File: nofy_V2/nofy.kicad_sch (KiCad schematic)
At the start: 144 parts, among them J10 Conn_01x01-Connector_Generic, J11 Conn_01x01-Connector_Generic, J12 Conn_01x01-Connector_Generic, J13 Conn_01x01-Connector_Generic, J14 Conn_01x01-Connector_Generic, J15 Conn_01x01-Connector_Generic, J16 Conn_01x01-Connector_Generic, J17 Conn_01x01-Connector_Generic, J18 Conn_01x01-Connector_Generic, J19 Conn_01x01-Connector_Generic, J20 Conn_01x01-Connector_Generic, J21 Conn_01x01-Connector_Generic, J22 PIn1x4, J23 PIn1x4, J24 PIn1x4, J25 PIn1x4, J26 PIn1x4, J27 PIn1x4, J28 PIn1x4, J29 PIn1x4, J30 PIn1x4, J31 PIn1x4, J32 PIn1x4, J33 PIn1x4, J34 PIn1x4, J35 PIn1x4, J36 PIn1x4, J37 PIn1x4, J38 PIn1x4, J39 PIn1x4, J40 PIn1x4, J41 PIn1x4, SW1 RotaryEncoder, SW10 SW_PUSH, SW11 SW_PUSH, SW12 SW_PUSH, SW13 SW_PUSH, SW14 SW_PUSH, SW15 SW_PUSH, SW16 SW_PUSH, SW17 SW_PUSH, SW18 SW_PUSH, SW19 SW_PUSH, SW2 RotaryEncoder, SW20 SW_PUSH, SW21 SW_PUSH, SW22 SW_PUSH, SW23 SW_PUSH, SW24 SW_PUSH, SW25 SW_PUSH, SW26 SW_PUSH, SW27 SW_PUSH, SW28 SW_PUSH, SW29 SW_PUSH, SW3 SW_SPDT, SW30 SW_PUSH, SW31 SW_PUSH, SW32 SW_PUSH, SW33 SW_PUSH, SW34 SW_PUSH, SW35 SW_PUSH, SW36 SW_PUSH, SW37 SW_PUSH, SW38 SW_PUSH, SW39 SW_PUSH, SW4 SW_SPDT, SW40 SW_PUSH, SW41 SW_PUSH, SW42 SW_PUSH, SW43 SW_PUSH, SW44 SW_PUSH, SW45 SW_PUSH, SW46 SW_PUSH, SW47 SW_PUSH, SW48 SW_PUSH, SW49 SW_PUSH, SW5 SW_PUSH, SW50 SW_PUSH, SW51 SW_PUSH, SW52 SW_PUSH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

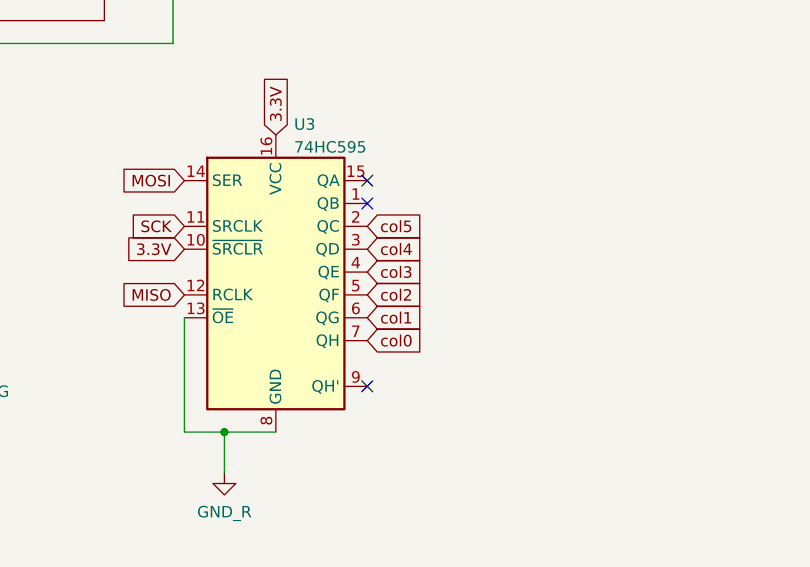
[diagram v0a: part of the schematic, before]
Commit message: Update : PCB
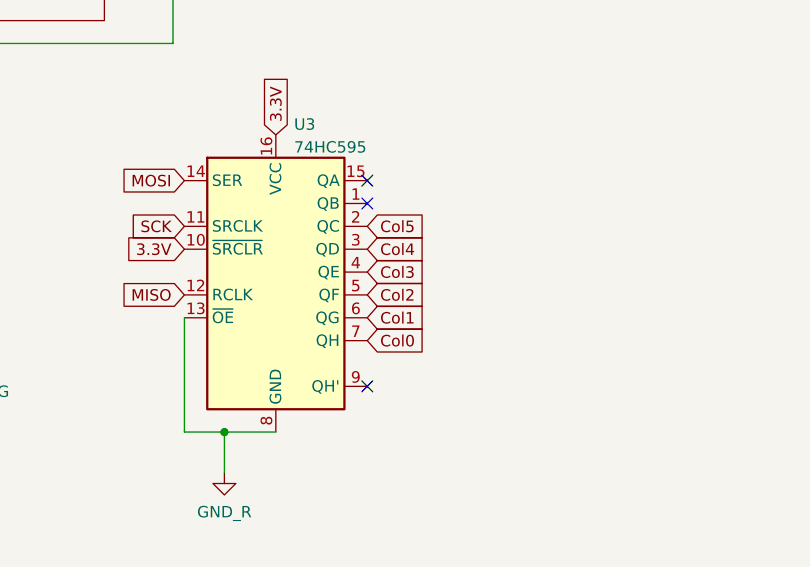
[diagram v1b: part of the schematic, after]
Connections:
- net col0 is gone; now on net Col0: U3.7 (QH)
- net col1 is gone; now on net Col1: U3.6 (QG)
- net col2 is gone; now on net Col2: U3.5 (QF)
- net col3 is gone; now on net Col3: U3.4 (QE)
- net col4 is gone; now on net Col4: U3.3 (QD)
- net col5 is gone; now on net Col5: U3.2 (QC)
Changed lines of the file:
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@@
 		)
 	)
-	(global_label "col0"
+	(global_label "Col0"
 		(shape input)
 		(at 119.38 107.95 0)
@@
 		)
 		(property "Intersheetrefs" "${INTERSHEET_REFS}"
-			(at 318.77 156.21 0)
-			(effects
-				(font
-					(size 1.27 1.27)
-				)
+			(at 126.6589 107.95 0)
+			(effects
+				(font
+					(size 1.27 1.27)
+				)
+				(justify left)
 				(hide yes)
 			)
@@
 		)
 	)
-	(global_label "col3"
+	(global_label "Col3"
 		(shape input)
 		(at 119.38 100.33 0)
@@
 		)
 		(property "Intersheetrefs" "${INTERSHEET_REFS}"
-			(at 318.77 156.21 0)
-			(effects
-				(font
-					(size 1.27 1.27)
-				)
+			(at 126.6589 100.33 0)
+			(effects
+				(font
+					(size 1.27 1.27)
+				)
+				(justify left)
 				(hide yes)
 			)
@@
 		)
 	)
-	(global_label "col1"
+	(global_label "Col1"
 		(shape input)
 		(at 119.38 105.41 0)
@@
 		)
 		(property "Intersheetrefs" "${INTERSHEET_REFS}"
-			(at 318.77 156.21 0)
-			(effects
-				(font
-					(size 1.27 1.27)
-				)
+			(at 126.6589 105.41 0)
+			(effects
+				(font
+					(size 1.27 1.27)
+				)
+				(justify left)
 				(hide yes)
 			)
@@
 		)
 	)
-	(global_label "col2"
+	(global_label "Col2"
 		(shape input)
 		(at 119.38 102.87 0)
@@
 		)
 		(property "Intersheetrefs" "${INTERSHEET_REFS}"
-			(at 318.77 156.21 0)
-			(effects
-				(font
-					(size 1.27 1.27)
-				)
+			(at 126.6589 102.87 0)
+			(effects
+				(font
+					(size 1.27 1.27)
+				)
+				(justify left)
 				(hide yes)
 			)
@@
 		)
 	)
-	(global_label "col4"
+	(global_label "Col4"
 		(shape input)
 		(at 119.38 97.79 0)
@@
 		)
 		(property "Intersheetrefs" "${INTERSHEET_REFS}"
-			(at 318.77 156.21 0)
-			(effects
-				(font
-					(size 1.27 1.27)
-				)
+			(at 126.6589 97.79 0)
+			(effects
+				(font
+					(size 1.27 1.27)
+				)
+				(justify left)
 				(hide yes)
 			)
@@
 		)
 	)
-	(global_label "col5"
+	(global_label "Col5"
 		(shape input)
 		(at 119.38 95.25 0)
@@
 		)
 		(property "Intersheetrefs" "${INTERSHEET_REFS}"
-			(at 318.77 156.21 0)
-			(effects
-				(font
-					(size 1.27 1.27)
-				)
-				(hide yes)
-			)
+			(at 126.6589 95.25 0)
+			(effects
+				(font
+					(size 1.27 1.27)
+				)
+				(justify left)
+				(hide yes)
+			)
